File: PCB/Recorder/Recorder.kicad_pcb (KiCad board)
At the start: 2 copper layers, 70 x 70 mm, 54 parts, among them J1 Battery, J2 Reset, J3 TC2030-USB-NL-DS, J4 TF_PUSH, J5 USB-C-Socket-H, Q2 CJ2301, SW1 SW_Push, U1 R, U2 L, U3 TP4054, U4 ME6211C33M5G-N, U5 MAX98357A, U6 ESP32-S3-MINI-1

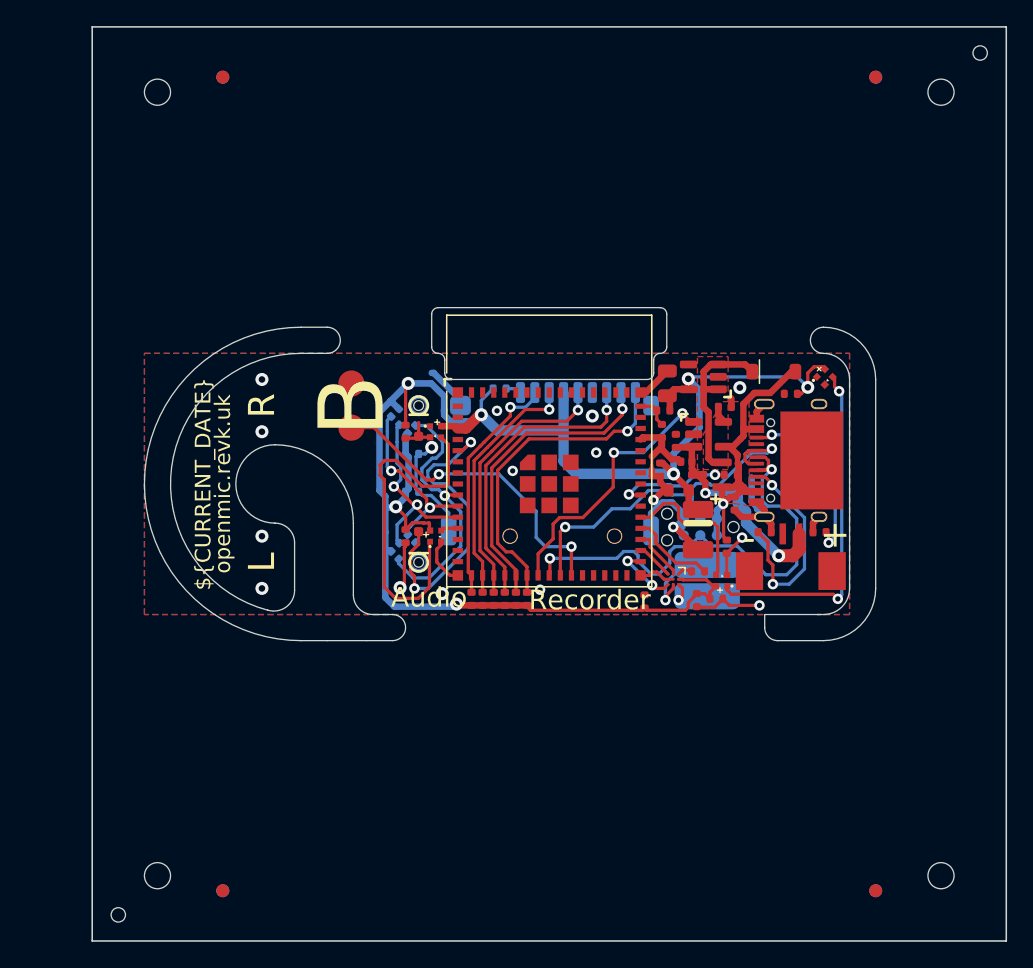
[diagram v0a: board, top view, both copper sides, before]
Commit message: Hook
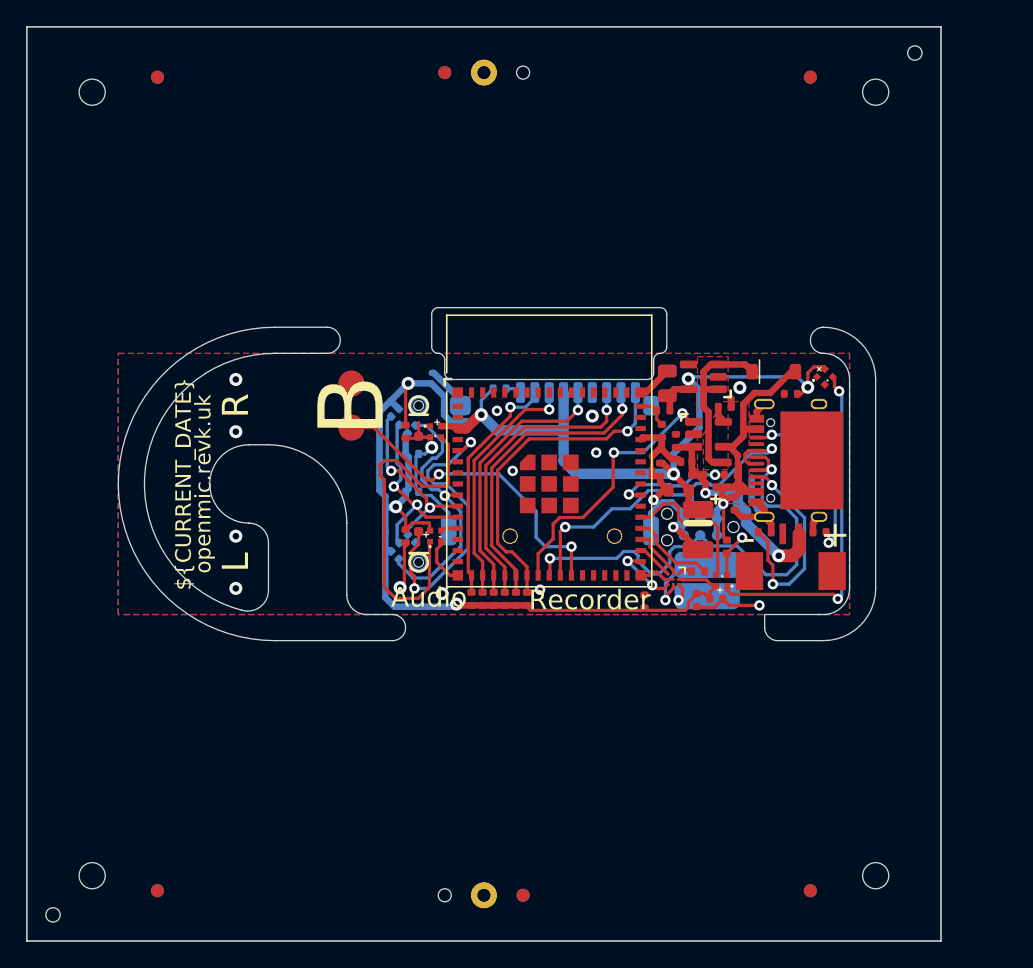
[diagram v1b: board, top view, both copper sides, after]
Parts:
- C12: renamed from C4; value 100nF -> 10uF
- C14: renamed from C12; value 10uF -> 100nF
- moved PCB1 5.00 mm to (95.0, 100.0)
- moved V1 5.00 mm to (95.0, 90.0)
- moved V2 5.00 mm to (95.0, 110.0)
- renumbered C14 to C4
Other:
- board text added: "41"
- board text removed: "37"
